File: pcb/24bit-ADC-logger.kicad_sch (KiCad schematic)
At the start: 21 parts, among them U1 REF5050AD, U2 ADS1232IPW, U3 TL071, U4 MAX15062A, U5 LP38693MP-5.0, U6 PicoW

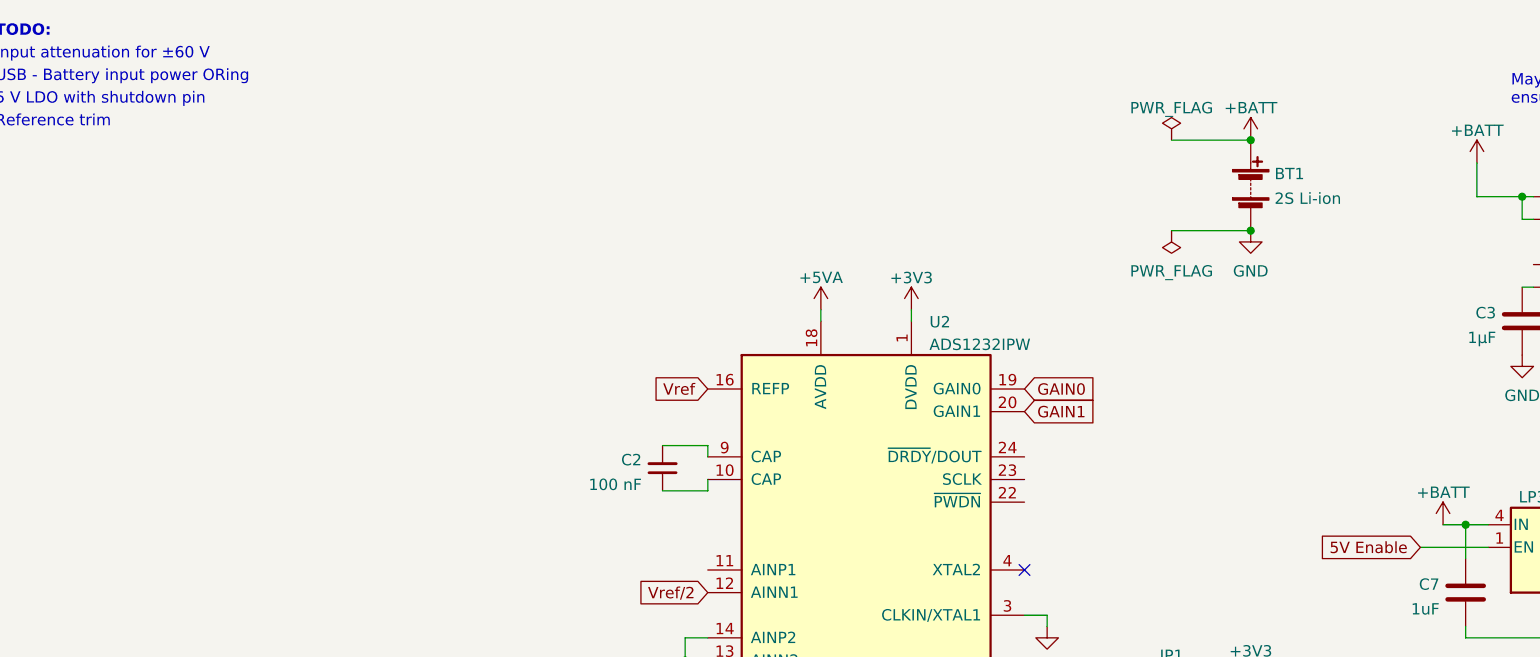
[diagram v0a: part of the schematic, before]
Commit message: test: move battery to trigger CI review diff
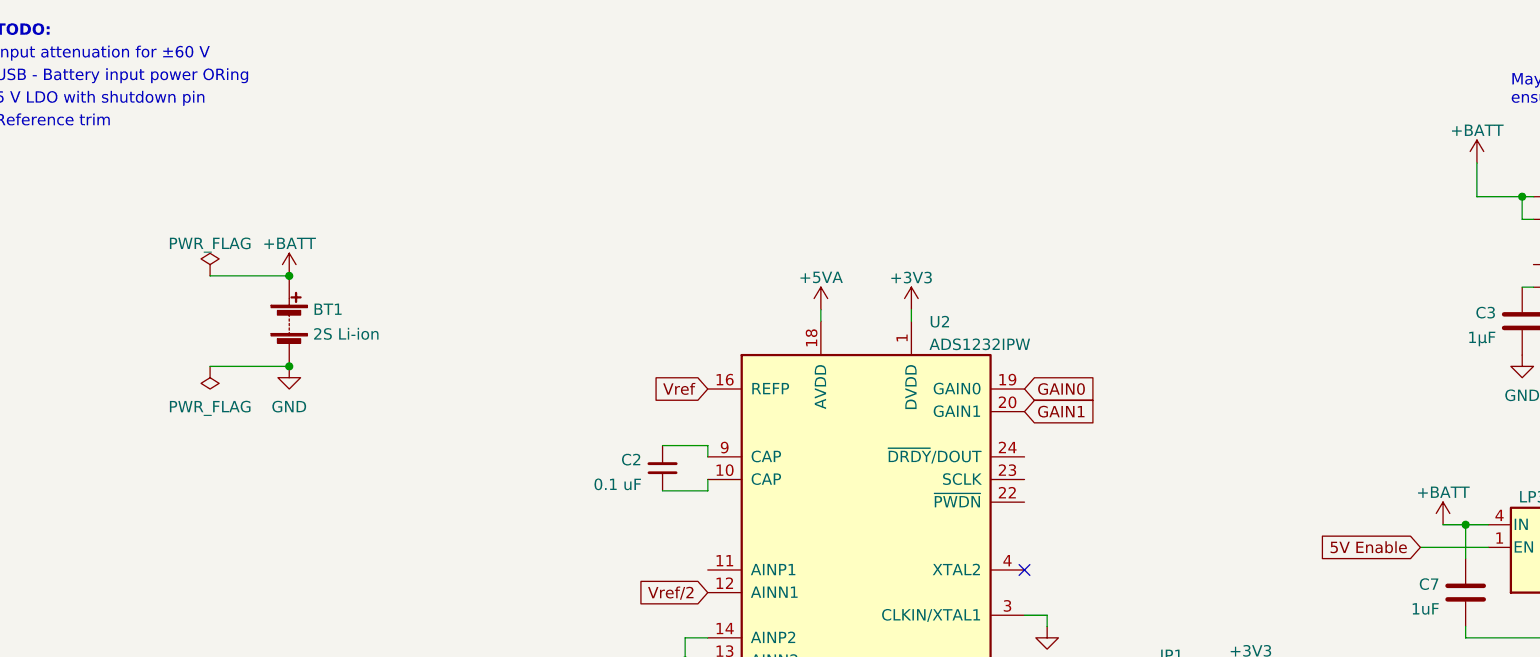
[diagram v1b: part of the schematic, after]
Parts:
- C2: value 100 nF -> 0.1 uF
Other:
- moved on the sheet: BT1
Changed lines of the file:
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@@
   (junction (at 207.01 73.66) (diameter 0) (color 0 0 0 0)
   )
-  (junction (at 157.48 40.64) (diameter 0) (color 0 0 0 0)
+  (junction (at 49.53 55.88) (diameter 0) (color 0 0 0 0)
   )
   (junction (at 259.08 111.76) (diameter 0) (color 0 0 0 0)
@@
   (junction (at 226.06 36.83) (diameter 0) (color 0 0 0 0)
   )
-  (junction (at 157.48 30.48) (diameter 0) (color 0 0 0 0)
+  (junction (at 49.53 45.72) (diameter 0) (color 0 0 0 0)
   )
   (junction (at 259.08 99.06) (diameter 0) (color 0 0 0 0)
@@
     (stroke (width 0) (type default) (color 0 0 0 0))
   )
-  (wire (pts (xy 148.59 30.48) (xy 157.48 30.48))
+  (wire (pts (xy 40.64 45.72) (xy 49.53 45.72))
     (stroke (width 0) (type default) (color 0 0 0 0))
   )
@@
     (stroke (width 0) (type default) (color 0 0 0 0))
   )
-  (wire (pts (xy 148.59 40.64) (xy 157.48 40.64))
+  (wire (pts (xy 40.64 55.88) (xy 49.53 55.88))
     (stroke (width 0) (type default) (color 0 0 0 0))
   )
@@
     (pin "1")
   )
-  (symbol (lib_id "power:PWR_FLAG") (at 148.59 30.48 0) (unit 1)
-    (in_bom yes) (on_board yes) (fields_autoplaced)
-    (property "Reference" "#FLG0101" (id 0) (at 148.59 28.575 0)
-      (effects (font (size 1.27 1.27)) hide)
-    )
-    (property "Value" "PWR_FLAG" (id 1) (at 148.59 26.8755 0))
-    (property "Footprint" "" (id 2) (at 148.59 30.48 0)
-      (effects (font (size 1.27 1.27)) hide)
-    )
-    (property "Datasheet" "~" (id 3) (at 148.59 30.48 0)
+  (symbol (lib_id "power:PWR_FLAG") (at 40.64 45.72 0) (unit 1)
+    (in_bom yes) (on_board yes) (fields_autoplaced)
+    (property "Reference" "#FLG0101" (id 0) (at 40.64 43.815 0)
+      (effects (font (size 1.27 1.27)) hide)
+    )
+    (property "Value" "PWR_FLAG" (id 1) (at 40.64 42.1155 0))
+    (property "Footprint" "" (id 2) (at 40.64 45.72 0)
+      (effects (font (size 1.27 1.27)) hide)
+    )
+    (property "Datasheet" "~" (id 3) (at 40.64 45.72 0)
       (effects (font (size 1.27 1.27)) hide)
     )
@@
     (pin "1")
   )
-  (symbol (lib_id "power:PWR_FLAG") (at 148.59 40.64 180) (unit 1)
-    (in_bom yes) (on_board yes) (fields_autoplaced)
-    (property "Reference" "#FLG01" (id 0) (at 148.59 42.545 0)
-      (effects (font (size 1.27 1.27)) hide)
-    )
-    (property "Value" "PWR_FLAG" (id 1) (at 148.59 45.2025 0))
-    (property "Footprint" "" (id 2) (at 148.59 40.64 0)
-      (effects (font (size 1.27 1.27)) hide)
-    )
-    (property "Datasheet" "~" (id 3) (at 148.59 40.64 0)
+  (symbol (lib_id "power:PWR_FLAG") (at 40.64 55.88 180) (unit 1)
+    (in_bom yes) (on_board yes) (fields_autoplaced)
+    (property "Reference" "#FLG01" (id 0) (at 40.64 57.785 0)
+      (effects (font (size 1.27 1.27)) hide)
+    )
+    (property "Value" "PWR_FLAG" (id 1) (at 40.64 60.4425 0))
+    (property "Footprint" "" (id 2) (at 40.64 55.88 0)
+      (effects (font (size 1.27 1.27)) hide)
+    )
+    (property "Datasheet" "~" (id 3) (at 40.64 55.88 0)
       (effects (font (size 1.27 1.27)) hide)
     )
@@
       (effects (font (size 1.27 1.27)) (justify right))
     )
-    (property "Value" "100 nF" (id 1) (at 89.1159 69.1702 0)
+    (property "Value" "0.1 uF" (id 1) (at 89.1159 69.1702 0)
       (effects (font (size 1.27 1.27)) (justify right))
     )
@@
     (pin "1")
   )
-  (symbol (lib_id "power:GND") (at 157.48 40.64 0) (unit 1)
-    (in_bom yes) (on_board yes) (fields_autoplaced)
-    (property "Reference" "#PWR02" (id 0) (at 157.48 46.99 0)
-      (effects (font (size 1.27 1.27)) hide)
-    )
-    (property "Value" "GND" (id 1) (at 157.48 45.2025 0))
-    (property "Footprint" "" (id 2) (at 157.48 40.64 0)
-      (effects (font (size 1.27 1.27)) hide)
-    )
-    (property "Datasheet" "" (id 3) (at 157.48 40.64 0)
+  (symbol (lib_id "power:GND") (at 49.53 55.88 0) (unit 1)
+    (in_bom yes) (on_board yes) (fields_autoplaced)
+    (property "Reference" "#PWR02" (id 0) (at 49.53 62.23 0)
+      (effects (font (size 1.27 1.27)) hide)
+    )
+    (property "Value" "GND" (id 1) (at 49.53 60.4425 0))
+    (property "Footprint" "" (id 2) (at 49.53 55.88 0)
+      (effects (font (size 1.27 1.27)) hide)
+    )
+    (property "Datasheet" "" (id 3) (at 49.53 55.88 0)
       (effects (font (size 1.27 1.27)) hide)
     )
@@
     (pin "9")
   )
-  (symbol (lib_id "Device:Battery") (at 157.48 35.56 0) (unit 1)
-    (in_bom yes) (on_board yes) (fields_autoplaced)
-    (property "Reference" "BT1" (id 0) (at 160.147 34.2705 0)
-      (effects (font (size 1.27 1.27)) (justify left))
-    )
-    (property "Value" "2S Li-ion" (id 1) (at 160.147 37.0456 0)
-      (effects (font (size 1.27 1.27)) (justify left))
-    )
-    (property "Footprint" "" (id 2) (at 157.48 34.036 90)
-      (effects (font (size 1.27 1.27)) hide)
-    )
-    (property "Datasheet" "~" (id 3) (at 157.48 34.036 90)
+  (symbol (lib_id "Device:Battery") (at 49.53 50.8 0) (unit 1)
+    (in_bom yes) (on_board yes) (fields_autoplaced)
+    (property "Reference" "BT1" (id 0) (at 52.197 49.5105 0)
+      (effects (font (size 1.27 1.27)) (justify left))
+    )
+    (property "Value" "2S Li-ion" (id 1) (at 52.197 52.2856 0)
+      (effects (font (size 1.27 1.27)) (justify left))
+    )
+    (property "Footprint" "" (id 2) (at 49.53 49.276 90)
+      (effects (font (size 1.27 1.27)) hide)
+    )
+    (property "Datasheet" "~" (id 3) (at 49.53 49.276 90)
       (effects (font (size 1.27 1.27)) hide)
     )
@@
     (pin "2")
   )
-  (symbol (lib_id "power:+BATT") (at 157.48 30.48 0) (unit 1)
-    (in_bom yes) (on_board yes) (fields_autoplaced)
-    (property "Reference" "#PWR01" (id 0) (at 157.48 34.29 0)
-      (effects (font (size 1.27 1.27)) hide)
-    )
-    (property "Value" "+BATT" (id 1) (at 157.48 26.8755 0))
-    (property "Footprint" "" (id 2) (at 157.48 30.48 0)
-      (effects (font (size 1.27 1.27)) hide)
-    )
-    (property "Datasheet" "" (id 3) (at 157.48 30.48 0)
+  (symbol (lib_id "power:+BATT") (at 49.53 45.72 0) (unit 1)
+    (in_bom yes) (on_board yes) (fields_autoplaced)
+    (property "Reference" "#PWR01" (id 0) (at 49.53 49.53 0)
+      (effects (font (size 1.27 1.27)) hide)
+    )
+    (property "Value" "+BATT" (id 1) (at 49.53 42.1155 0))
+    (property "Footprint" "" (id 2) (at 49.53 45.72 0)
+      (effects (font (size 1.27 1.27)) hide)
+    )
+    (property "Datasheet" "" (id 3) (at 49.53 45.72 0)
       (effects (font (size 1.27 1.27)) hide)
     )
@@
     )
     (path "/0fafedb4-75f0-46bd-ad25-e71605789522"
-      (reference "C2") (unit 1) (value "100 nF") (footprint "")
+      (reference "C2") (unit 1) (value "0.1 uF") (footprint "")
     )
     (path "/c2d5842f-85a0-468a-8cc5-d2ab1d5f7796"

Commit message: Revert "test: move battery to trigger CI review diff"
This reverts commit 0879a356b85a0944c1810179dfdc8ad8240099bf.
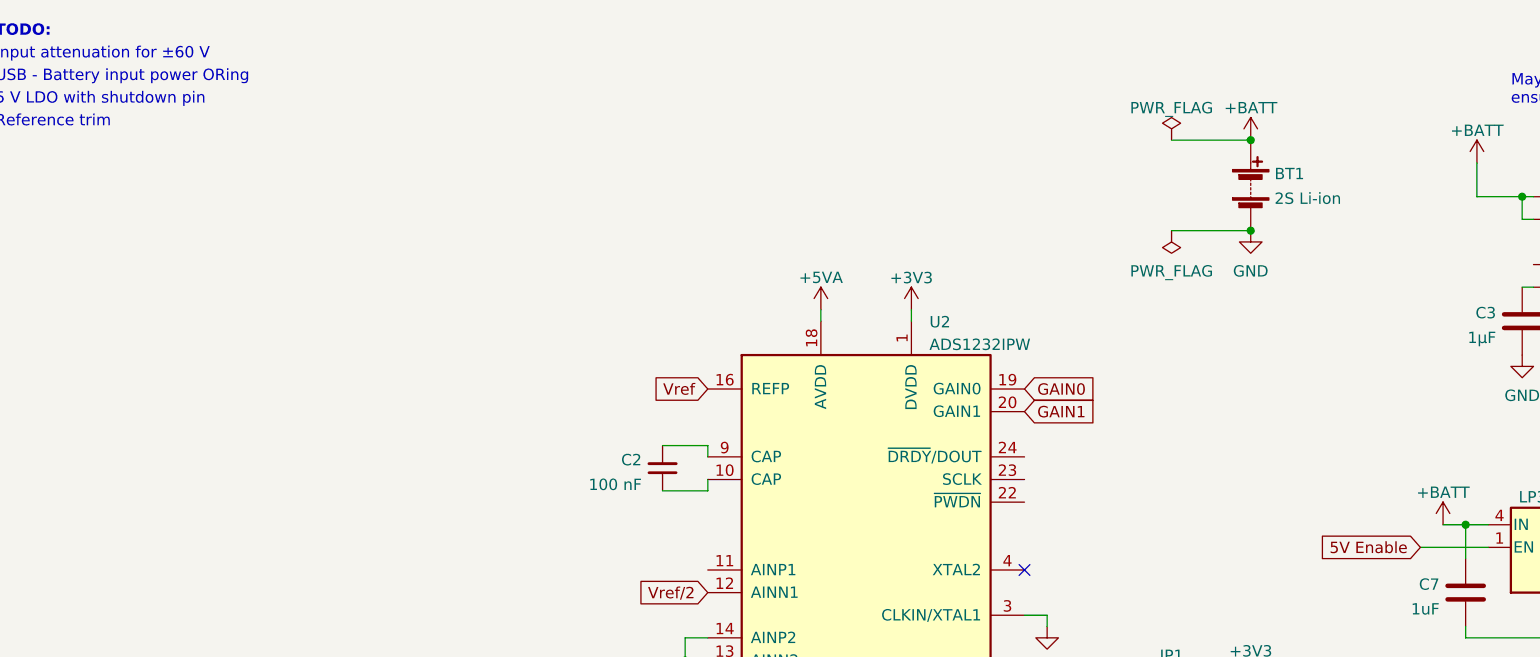
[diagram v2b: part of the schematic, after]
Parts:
- C2: value 0.1 uF -> 100 nF
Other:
- moved on the sheet: BT1
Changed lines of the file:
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@@
   (junction (at 207.01 73.66) (diameter 0) (color 0 0 0 0)
   )
-  (junction (at 49.53 55.88) (diameter 0) (color 0 0 0 0)
+  (junction (at 157.48 40.64) (diameter 0) (color 0 0 0 0)
   )
   (junction (at 259.08 111.76) (diameter 0) (color 0 0 0 0)
@@
   (junction (at 226.06 36.83) (diameter 0) (color 0 0 0 0)
   )
-  (junction (at 49.53 45.72) (diameter 0) (color 0 0 0 0)
+  (junction (at 157.48 30.48) (diameter 0) (color 0 0 0 0)
   )
   (junction (at 259.08 99.06) (diameter 0) (color 0 0 0 0)
@@
     (stroke (width 0) (type default) (color 0 0 0 0))
   )
-  (wire (pts (xy 40.64 45.72) (xy 49.53 45.72))
+  (wire (pts (xy 148.59 30.48) (xy 157.48 30.48))
     (stroke (width 0) (type default) (color 0 0 0 0))
   )
@@
     (stroke (width 0) (type default) (color 0 0 0 0))
   )
-  (wire (pts (xy 40.64 55.88) (xy 49.53 55.88))
+  (wire (pts (xy 148.59 40.64) (xy 157.48 40.64))
     (stroke (width 0) (type default) (color 0 0 0 0))
   )
@@
     (pin "1")
   )
-  (symbol (lib_id "power:PWR_FLAG") (at 40.64 45.72 0) (unit 1)
-    (in_bom yes) (on_board yes) (fields_autoplaced)
-    (property "Reference" "#FLG0101" (id 0) (at 40.64 43.815 0)
-      (effects (font (size 1.27 1.27)) hide)
-    )
-    (property "Value" "PWR_FLAG" (id 1) (at 40.64 42.1155 0))
-    (property "Footprint" "" (id 2) (at 40.64 45.72 0)
-      (effects (font (size 1.27 1.27)) hide)
-    )
-    (property "Datasheet" "~" (id 3) (at 40.64 45.72 0)
+  (symbol (lib_id "power:PWR_FLAG") (at 148.59 30.48 0) (unit 1)
+    (in_bom yes) (on_board yes) (fields_autoplaced)
+    (property "Reference" "#FLG0101" (id 0) (at 148.59 28.575 0)
+      (effects (font (size 1.27 1.27)) hide)
+    )
+    (property "Value" "PWR_FLAG" (id 1) (at 148.59 26.8755 0))
+    (property "Footprint" "" (id 2) (at 148.59 30.48 0)
+      (effects (font (size 1.27 1.27)) hide)
+    )
+    (property "Datasheet" "~" (id 3) (at 148.59 30.48 0)
       (effects (font (size 1.27 1.27)) hide)
     )
@@
     (pin "1")
   )
-  (symbol (lib_id "power:PWR_FLAG") (at 40.64 55.88 180) (unit 1)
-    (in_bom yes) (on_board yes) (fields_autoplaced)
-    (property "Reference" "#FLG01" (id 0) (at 40.64 57.785 0)
-      (effects (font (size 1.27 1.27)) hide)
-    )
-    (property "Value" "PWR_FLAG" (id 1) (at 40.64 60.4425 0))
-    (property "Footprint" "" (id 2) (at 40.64 55.88 0)
-      (effects (font (size 1.27 1.27)) hide)
-    )
-    (property "Datasheet" "~" (id 3) (at 40.64 55.88 0)
+  (symbol (lib_id "power:PWR_FLAG") (at 148.59 40.64 180) (unit 1)
+    (in_bom yes) (on_board yes) (fields_autoplaced)
+    (property "Reference" "#FLG01" (id 0) (at 148.59 42.545 0)
+      (effects (font (size 1.27 1.27)) hide)
+    )
+    (property "Value" "PWR_FLAG" (id 1) (at 148.59 45.2025 0))
+    (property "Footprint" "" (id 2) (at 148.59 40.64 0)
+      (effects (font (size 1.27 1.27)) hide)
+    )
+    (property "Datasheet" "~" (id 3) (at 148.59 40.64 0)
       (effects (font (size 1.27 1.27)) hide)
     )
@@
       (effects (font (size 1.27 1.27)) (justify right))
     )
-    (property "Value" "0.1 uF" (id 1) (at 89.1159 69.1702 0)
+    (property "Value" "100 nF" (id 1) (at 89.1159 69.1702 0)
       (effects (font (size 1.27 1.27)) (justify right))
     )
@@
     (pin "1")
   )
-  (symbol (lib_id "power:GND") (at 49.53 55.88 0) (unit 1)
-    (in_bom yes) (on_board yes) (fields_autoplaced)
-    (property "Reference" "#PWR02" (id 0) (at 49.53 62.23 0)
-      (effects (font (size 1.27 1.27)) hide)
-    )
-    (property "Value" "GND" (id 1) (at 49.53 60.4425 0))
-    (property "Footprint" "" (id 2) (at 49.53 55.88 0)
-      (effects (font (size 1.27 1.27)) hide)
-    )
-    (property "Datasheet" "" (id 3) (at 49.53 55.88 0)
+  (symbol (lib_id "power:GND") (at 157.48 40.64 0) (unit 1)
+    (in_bom yes) (on_board yes) (fields_autoplaced)
+    (property "Reference" "#PWR02" (id 0) (at 157.48 46.99 0)
+      (effects (font (size 1.27 1.27)) hide)
+    )
+    (property "Value" "GND" (id 1) (at 157.48 45.2025 0))
+    (property "Footprint" "" (id 2) (at 157.48 40.64 0)
+      (effects (font (size 1.27 1.27)) hide)
+    )
+    (property "Datasheet" "" (id 3) (at 157.48 40.64 0)
       (effects (font (size 1.27 1.27)) hide)
     )
@@
     (pin "9")
   )
-  (symbol (lib_id "Device:Battery") (at 49.53 50.8 0) (unit 1)
-    (in_bom yes) (on_board yes) (fields_autoplaced)
-    (property "Reference" "BT1" (id 0) (at 52.197 49.5105 0)
-      (effects (font (size 1.27 1.27)) (justify left))
-    )
-    (property "Value" "2S Li-ion" (id 1) (at 52.197 52.2856 0)
-      (effects (font (size 1.27 1.27)) (justify left))
-    )
-    (property "Footprint" "" (id 2) (at 49.53 49.276 90)
-      (effects (font (size 1.27 1.27)) hide)
-    )
-    (property "Datasheet" "~" (id 3) (at 49.53 49.276 90)
+  (symbol (lib_id "Device:Battery") (at 157.48 35.56 0) (unit 1)
+    (in_bom yes) (on_board yes) (fields_autoplaced)
+    (property "Reference" "BT1" (id 0) (at 160.147 34.2705 0)
+      (effects (font (size 1.27 1.27)) (justify left))
+    )
+    (property "Value" "2S Li-ion" (id 1) (at 160.147 37.0456 0)
+      (effects (font (size 1.27 1.27)) (justify left))
+    )
+    (property "Footprint" "" (id 2) (at 157.48 34.036 90)
+      (effects (font (size 1.27 1.27)) hide)
+    )
+    (property "Datasheet" "~" (id 3) (at 157.48 34.036 90)
       (effects (font (size 1.27 1.27)) hide)
     )
@@
     (pin "2")
   )
-  (symbol (lib_id "power:+BATT") (at 49.53 45.72 0) (unit 1)
-    (in_bom yes) (on_board yes) (fields_autoplaced)
-    (property "Reference" "#PWR01" (id 0) (at 49.53 49.53 0)
-      (effects (font (size 1.27 1.27)) hide)
-    )
-    (property "Value" "+BATT" (id 1) (at 49.53 42.1155 0))
-    (property "Footprint" "" (id 2) (at 49.53 45.72 0)
-      (effects (font (size 1.27 1.27)) hide)
-    )
-    (property "Datasheet" "" (id 3) (at 49.53 45.72 0)
+  (symbol (lib_id "power:+BATT") (at 157.48 30.48 0) (unit 1)
+    (in_bom yes) (on_board yes) (fields_autoplaced)
+    (property "Reference" "#PWR01" (id 0) (at 157.48 34.29 0)
+      (effects (font (size 1.27 1.27)) hide)
+    )
+    (property "Value" "+BATT" (id 1) (at 157.48 26.8755 0))
+    (property "Footprint" "" (id 2) (at 157.48 30.48 0)
+      (effects (font (size 1.27 1.27)) hide)
+    )
+    (property "Datasheet" "" (id 3) (at 157.48 30.48 0)
       (effects (font (size 1.27 1.27)) hide)
     )
@@
     )
     (path "/0fafedb4-75f0-46bd-ad25-e71605789522"
-      (reference "C2") (unit 1) (value "0.1 uF") (footprint "")
+      (reference "C2") (unit 1) (value "100 nF") (footprint "")
     )
     (path "/c2d5842f-85a0-468a-8cc5-d2ab1d5f7796"
